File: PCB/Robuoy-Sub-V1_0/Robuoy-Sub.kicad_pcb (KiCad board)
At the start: 4 copper layers, 160 x 160 mm, 117 parts, among them J101 PROG/JTAG, J102 TO PUSH BUTTON, J103 ESC_BB, J104 ESC_SB, J105 RS232_Option, J106 Compass, J201 Accu, J202 LoadbalanceAccu1, J203 LoadbalanceAccu2, J204 Conn_01x10, J205 PWR_Charger, J206 LoadbalanceCharger, J207 ESCSB, J208 ESCBB, Q101 AO3400A, Q201 AO3400A, Q202 AO3400A, Q203 AO3400A, Q204 AO3400A, Q205 AO3400A, Q206 AO3400A, Q207 AO3400A, Q208 AO3400A, SW101 ~{BOOT}, SW102 ~{RESET}, SW201 SS-12D11-G050/On-Off, U101 ESP32-WROOM-32E_(visible_peri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, U102 USBLC6-4SC6, U103 LTC4311, U104 SN74LV1T34DBV, U105 SN74LV1T34DBV, U201 TPS5430DDAR, U202 SN74LV1T34DBV, U203 SN74LV1T34DBV, U204 TLV61046ADB

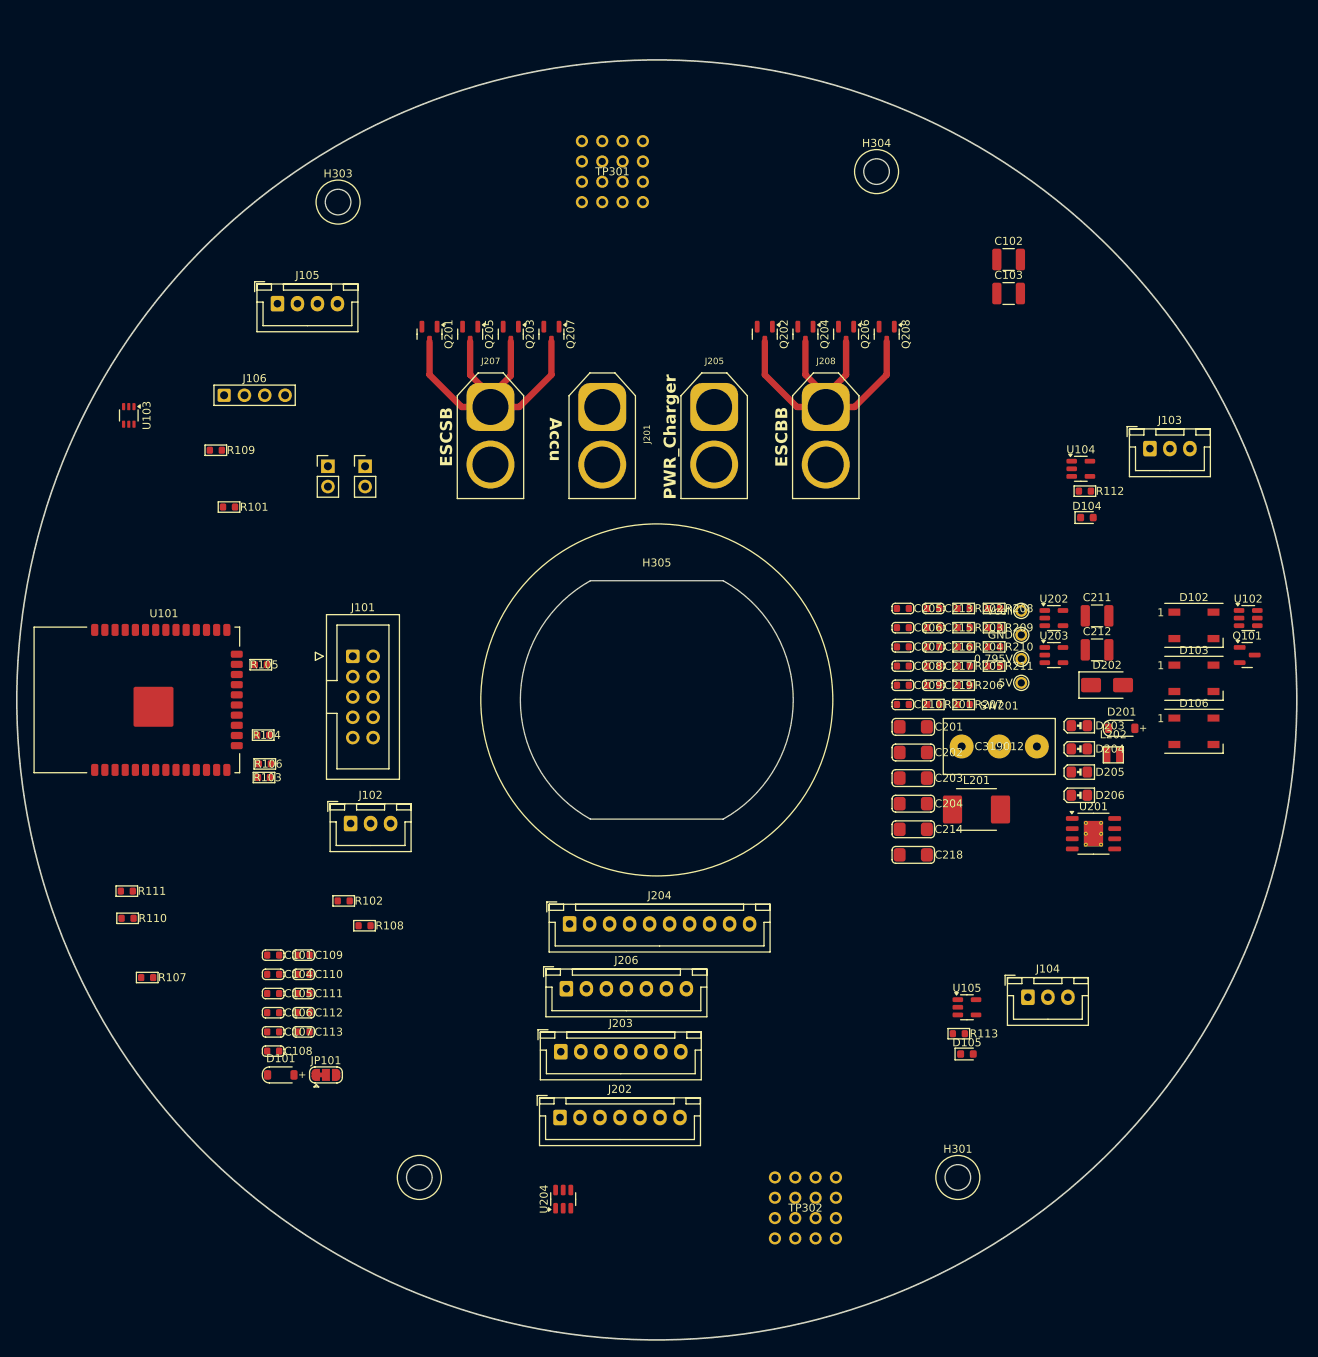
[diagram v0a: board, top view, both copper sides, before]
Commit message: Sub PCB parts okay
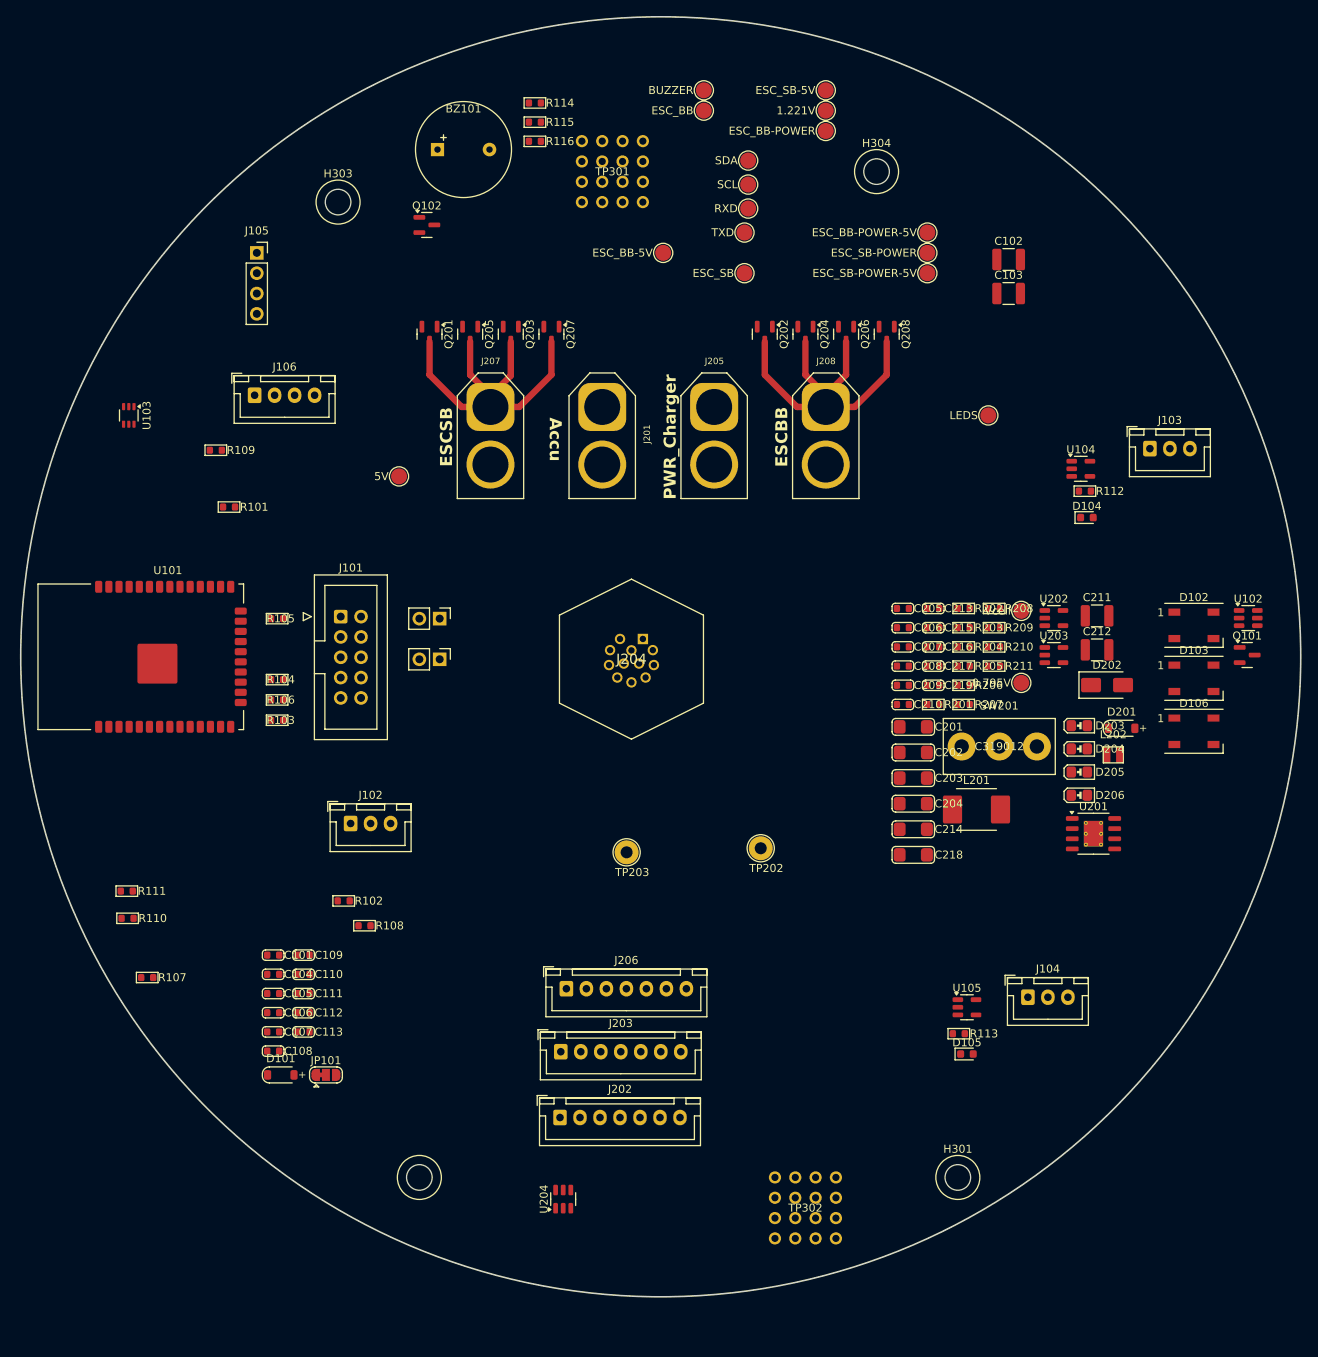
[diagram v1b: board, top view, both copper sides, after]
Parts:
- removed H305: GX16_CutOut, A_Mechanical:GX16_CutOut
- added BZ101: Buzzer, A_Misc:Buzzer-12x6.5x5.2, F.Cu at (70.3, 46.6)
- added Q102: AO3400A, Package_TO_SOT_SMD:SOT-23, F.Cu at (65.8, 56.0)
- added R114: 100, A_Device:R_0603, F.Cu at (79.3, 40.8)
- added R115: 100, A_Device:R_0603, F.Cu at (79.3, 43.2)
- added R116: 100, A_Device:R_0603, F.Cu at (79.3, 45.6)
- added TP101: BUZZER, A_Pads_Pins:Testpad_2, F.Cu at (100.4, 39.2)
- added TP102: ESC_BB, A_Pads_Pins:Testpad_2, F.Cu at (100.4, 41.7)
- added TP103: ESC_SB, A_Pads_Pins:Testpad_2, F.Cu at (105.5, 62.0)
- added TP104: LEDS, A_Pads_Pins:Testpad_2, F.Cu at (135.9, 79.8)
- added TP105: ESC_BB-5V, A_Pads_Pins:Testpad_2, F.Cu at (95.3, 59.5)
- added TP106: ESC_SB-5V, A_Pads_Pins:Testpad_2, F.Cu at (115.6, 39.2)
- added TP107: SDA, A_Pads_Pins:Testpad_2, F.Cu at (105.9, 48.0)
- added TP108: SCL, A_Pads_Pins:Testpad_2, F.Cu at (105.9, 51.0)
- added TP109: RXD, A_Pads_Pins:Testpad_2, F.Cu at (105.9, 54.0)
- added TP110: TXD, A_Pads_Pins:Testpad_2, F.Cu at (105.5, 57.0)
- added TP205: 5V, A_Pads_Pins:Testpad_2, F.Cu at (62.3, 87.5)
- added TP206: 1.221V, A_Pads_Pins:Testpad_2, F.Cu at (115.6, 41.7)
- added TP207: ESC_BB-POWER, A_Pads_Pins:Testpad_2, F.Cu at (115.6, 44.3)
- added TP208: ESC_SB-POWER, A_Pads_Pins:Testpad_2, F.Cu at (128.3, 59.5)
- added TP209: ESC_BB-POWER-5V, A_Pads_Pins:Testpad_2, F.Cu at (128.3, 57.0)
- added TP210: ESC_SB-POWER-5V, A_Pads_Pins:Testpad_2, F.Cu at (128.3, 62.0)
- J102: value TO PUSH BUTTON -> PUSH BUTTON
- J105: footprint Connector_JST:JST_XH_B4B-XH-A_1x04_P2.50mm_Vertical -> Connector_PinSocket_2.54mm:PinSocket_1x04_P2.54mm_Vertical
- J106: footprint A_Connector:Header_1x04_P2.54_Male -> Connector_JST:JST_XH_B4B-XH-A_1x04_P2.50mm_Vertical
- J204: value Conn_01x10 -> CHARGE/ON-OFF; footprint Connector_JST:JST_XH_B10B-XH-A_1x10_P2.50mm_Vertical -> A_Connector:T4140012121000
- TP201: footprint A_Pads_Pins:Testpoint_0.9x1.5 -> A_Pads_Pins:Testpad_2
- TP202: footprint A_Pads_Pins:Testpoint_0.9x1.5 -> TestPoint:TestPoint_Loop_D2.54mm_Drill1.5mm_Beaded
- TP203: value 0.795V -> GND; footprint A_Pads_Pins:Testpoint_0.9x1.5 -> TestPoint:TestPoint_Loop_D2.54mm_Drill1.5mm_Beaded
- TP204: value 5V -> 0.795V; footprint A_Pads_Pins:Testpoint_0.9x1.5 -> A_Pads_Pins:Testpad_2
- moved TP203 54.9 mm to (90.7, 134.4)
- moved TP202 42.1 mm to (107.5, 133.9)
- moved J204 36.8 mm to (92.8, 107.8)
- moved SW101 27.9 mm to (67.4, 110.3), turned to -90 degrees
- moved SW102 21.2 mm to (67.4, 105.2), turned to -90 degrees
- moved R106 8.15 mm to (47.0, 115.4)
- moved R103 7.35 mm to (47.0, 117.9)
- moved R104 7.15 mm to (47.0, 112.8)
- moved J105 6.85 mm to (44.5, 59.5)
- moved R105 6.11 mm to (47.0, 105.2)
- moved U101 5.41 mm to (30.0, 110.0)
- moved J101 5.18 mm to (55.0, 105.0)
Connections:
- J103 pad 3: GND -> Net-(J103-Pin_3)
- J104 pad 3: GND -> Net-(J104-Pin_3)
- J204 pad 10: Vbatt -> GND
- TP203 pad 1: Net-(U204-FB) -> GND
- TP204 pad 1: +5V -> Net-(U204-FB)
- U101 pad 26: unconnected-(U101-D1/GPIO4-Pad26) -> BUZZER
